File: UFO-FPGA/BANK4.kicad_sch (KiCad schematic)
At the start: 19 parts, among them J6 Conn_02x02_Counter_Clockwise, U1 ICE40HX8K-BG121, U9 N25Q032A13ESC40F

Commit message: pcb 0603
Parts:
- C15, C16, C17, C20: footprint Capacitor_SMD:C_0805_2012Metric_Pad1.18x1.45mm_HandSolder -> Capacitor_SMD:C_0603_1608Metric_Pad1.08x0.95mm_HandSolder
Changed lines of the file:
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@@
       (effects (font (size 1.27 1.27)) (justify left))
     )
-    (property "Footprint" "Capacitor_SMD:C_0805_2012Metric_Pad1.18x1.45mm_HandSolder" (at 169.8752 81.28 0)
+    (property "Footprint" "Capacitor_SMD:C_0603_1608Metric_Pad1.08x0.95mm_HandSolder" (at 169.8752 81.28 0)
       (effects (font (size 1.27 1.27)) hide)
     )
@@
       (effects (font (size 1.27 1.27)) (justify left))
     )
-    (property "Footprint" "Capacitor_SMD:C_0805_2012Metric_Pad1.18x1.45mm_HandSolder" (at 84.7852 71.12 0)
+    (property "Footprint" "Capacitor_SMD:C_0603_1608Metric_Pad1.08x0.95mm_HandSolder" (at 84.7852 71.12 0)
       (effects (font (size 1.27 1.27)) hide)
     )
@@
       (effects (font (size 1.27 1.27)) (justify left))
     )
-    (property "Footprint" "Capacitor_SMD:C_0805_2012Metric_Pad1.18x1.45mm_HandSolder" (at 84.7852 81.28 0)
+    (property "Footprint" "Capacitor_SMD:C_0603_1608Metric_Pad1.08x0.95mm_HandSolder" (at 84.7852 81.28 0)
       (effects (font (size 1.27 1.27)) hide)
     )
@@
       (effects (font (size 1.27 1.27)) (justify left))
     )
-    (property "Footprint" "Capacitor_SMD:C_0805_2012Metric_Pad1.18x1.45mm_HandSolder" (at 131.7752 57.15 0)
-      (effects (font (size 1.27 1.27)) hide)
-    )
+    (property "Footprint" "Capacitor_SMD:C_0603_1608Metric_Pad1.08x0.95mm_HandSolder" (at 131.7752 57.15 0)
+      (effects (font (size 1.27 1.27)) hide)
+    )

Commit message: 0603
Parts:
- R21, R22, R23, R24: footprint Resistor_SMD:R_0805_2012Metric_Pad1.20x1.40mm_HandSolder -> Resistor_SMD:R_0603_1608Metric_Pad0.98x0.95mm_HandSolder
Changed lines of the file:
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@@
       (effects (font (size 1.27 1.27)) (justify left))
     )
-    (property "Footprint" "Resistor_SMD:R_0805_2012Metric_Pad1.20x1.40mm_HandSolder" (at 211.582 60.96 90)
+    (property "Footprint" "Resistor_SMD:R_0603_1608Metric_Pad0.98x0.95mm_HandSolder" (at 211.582 60.96 90)
       (effects (font (size 1.27 1.27)) hide)
     )
@@
       (effects (font (size 1.27 1.27)) (justify left))
     )
-    (property "Footprint" "Resistor_SMD:R_0805_2012Metric_Pad1.20x1.40mm_HandSolder" (at 219.202 60.96 90)
+    (property "Footprint" "Resistor_SMD:R_0603_1608Metric_Pad0.98x0.95mm_HandSolder" (at 219.202 60.96 90)
       (effects (font (size 1.27 1.27)) hide)
     )
@@
       (effects (font (size 1.27 1.27)) (justify left))
     )
-    (property "Footprint" "Resistor_SMD:R_0805_2012Metric_Pad1.20x1.40mm_HandSolder" (at 203.962 60.96 90)
+    (property "Footprint" "Resistor_SMD:R_0603_1608Metric_Pad0.98x0.95mm_HandSolder" (at 203.962 60.96 90)
       (effects (font (size 1.27 1.27)) hide)
     )
@@
       (effects (font (size 1.27 1.27)) (justify left))
     )
-    (property "Footprint" "Resistor_SMD:R_0805_2012Metric_Pad1.20x1.40mm_HandSolder" (at 145.542 53.34 90)
-      (effects (font (size 1.27 1.27)) hide)
-    )
+    (property "Footprint" "Resistor_SMD:R_0603_1608Metric_Pad0.98x0.95mm_HandSolder" (at 145.542 53.34 90)
+      (effects (font (size 1.27 1.27)) hide)
+    )

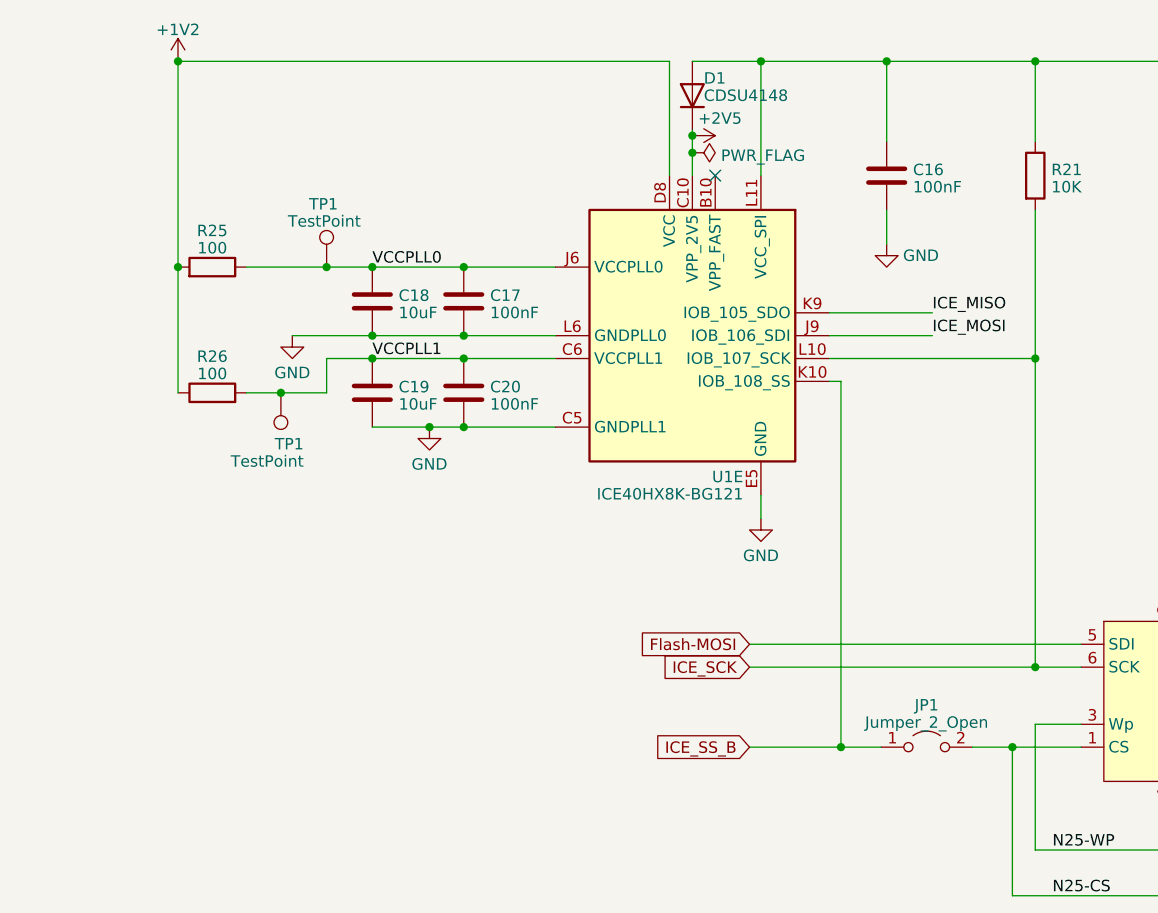
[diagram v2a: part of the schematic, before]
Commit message: pcb
added John zendong
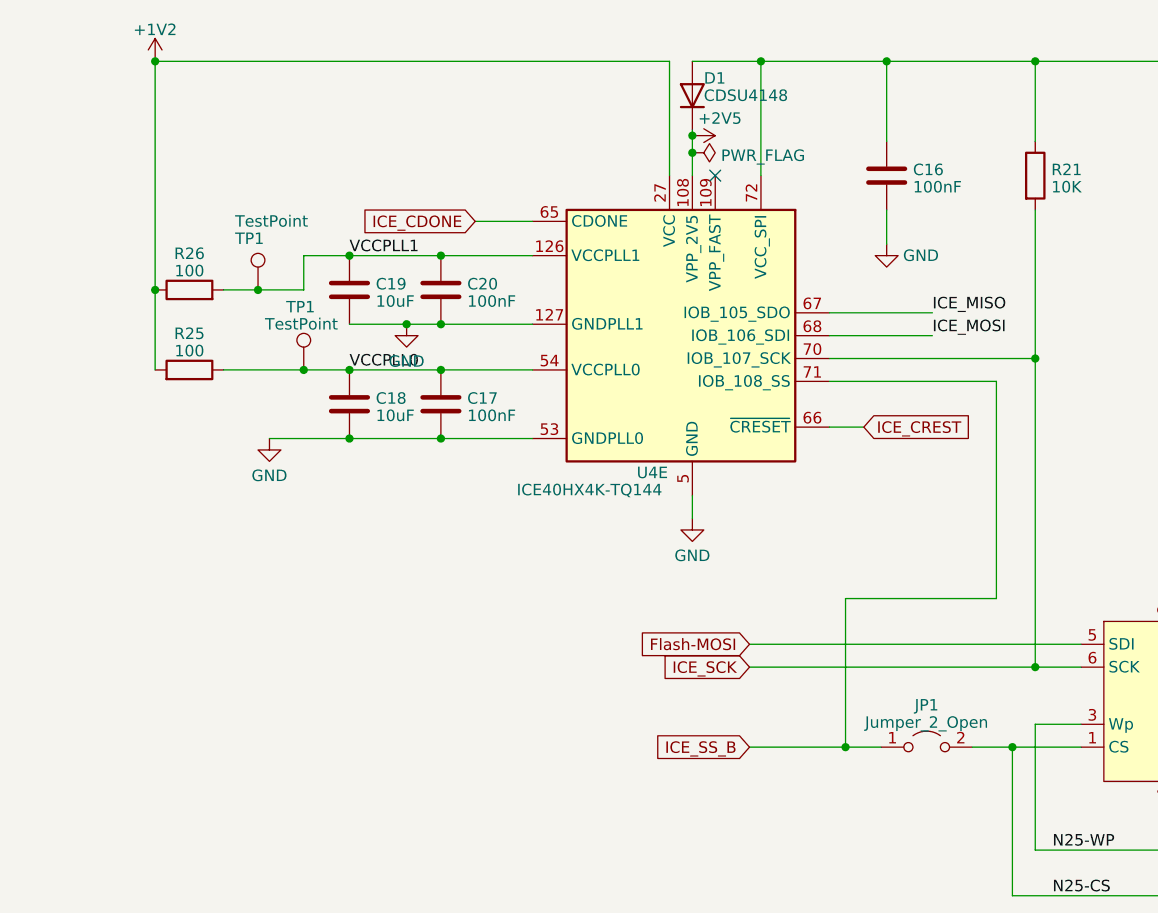
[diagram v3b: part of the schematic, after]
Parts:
- removed U1: ICE40HX8K-BG121, Package_BGA:BGA-121_9.0x9.0mm_Layout11x11_P0.8mm_Ball0.4mm_Pad0.35mm_NSMD, symbol FPGA_Lattice:ICE40HX8K-BG121
- added U4: ICE40HX4K-TQ144, Package_QFP:TQFP-144_20x20mm_P0.5mm, symbol FPGA_Lattice:ICE40HX4K-TQ144
- J6: footprint Connector_PinHeader_2.54mm:PinHeader_2x02_P2.54mm_Vertical -> Connector_PinHeader_1.27mm:PinHeader_2x02_P1.27mm_Vertical
- JP1: footprint Connector_PinHeader_2.54mm:PinHeader_1x02_P2.54mm_Vertical -> Connector_PinHeader_1.27mm:PinHeader_1x02_P1.27mm_Vertical
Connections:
- net +1V2: now also U4.111 (VCC), U4.27 (VCC), U4.40 (VCC), U4.92 (VCC)
- net +2V5: now also U4.108 (VPP_2V5)
- net +3V3: now also U4.72 (VCC_SPI)
- net GND: now also U4.103 (GND), U4.127 (GNDPLL1), U4.13 (GND), U4.132 (GND), U4.14 (GND), U4.140 (GND), U4.5 (GND), U4.53 (GNDPLL0), U4.59 (GND), U4.69 (GND), U4.86 (GND)
- net ICE_MISO: now also U4.67 (IOB_105_SDO)
- net ICE_MOSI: now also U4.68 (IOB_106_SDI)
- net ICE_SCK: now also U4.70 (IOB_107_SCK)
- net ICE_SS_B: now also U4.71 (IOB_108_SS)
- net VCCPLL0: now also U4.54 (VCCPLL0)
- net VCCPLL1: now also U4.126 (VCCPLL1)
- new net ICE_CDONE: U4.65 (CDONE)
- new net ICE_CREST: U4.66 (~{CRESET})
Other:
- moved on the sheet: C17, C18, C19, C20, R25, R26, TP1
